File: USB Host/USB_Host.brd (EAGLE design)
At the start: 35 x 64 mm, 6 parts, among them J3 DIN5, X1 PG203J

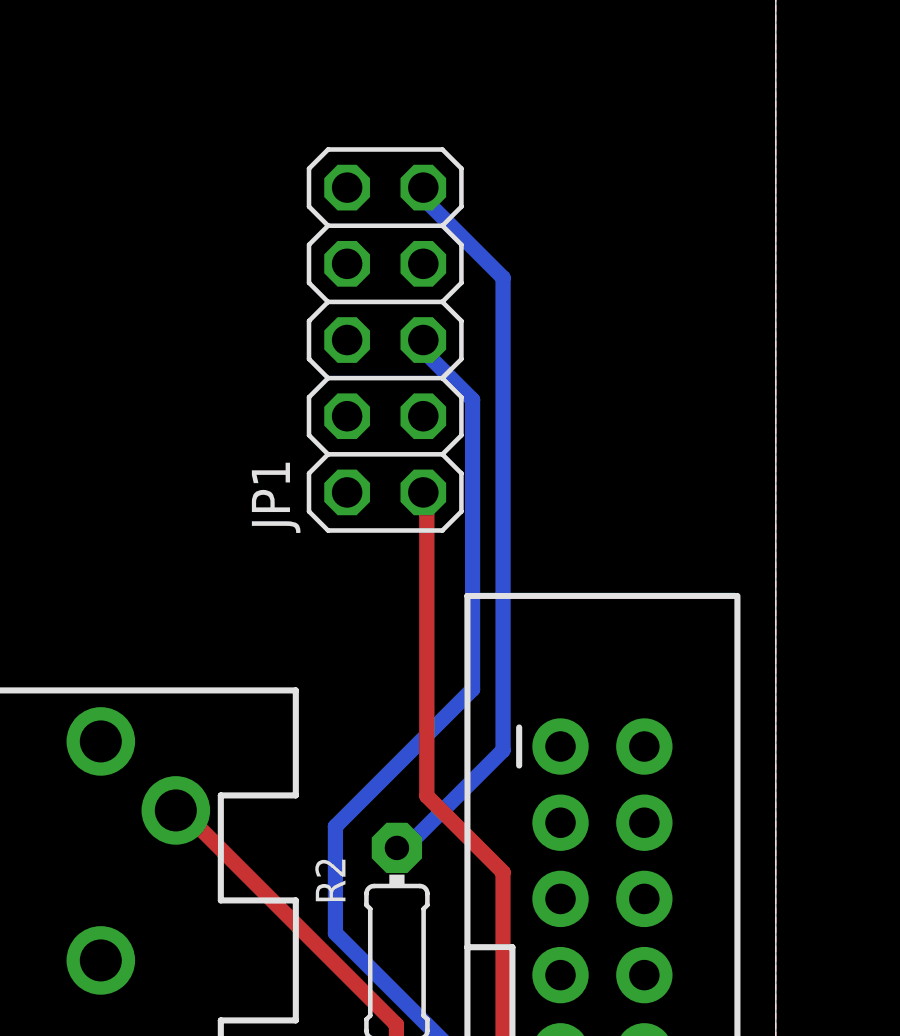
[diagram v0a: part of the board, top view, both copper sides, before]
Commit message: Adjustments to PCB Signed-off-by: goslo <digit99@mailinator.com>
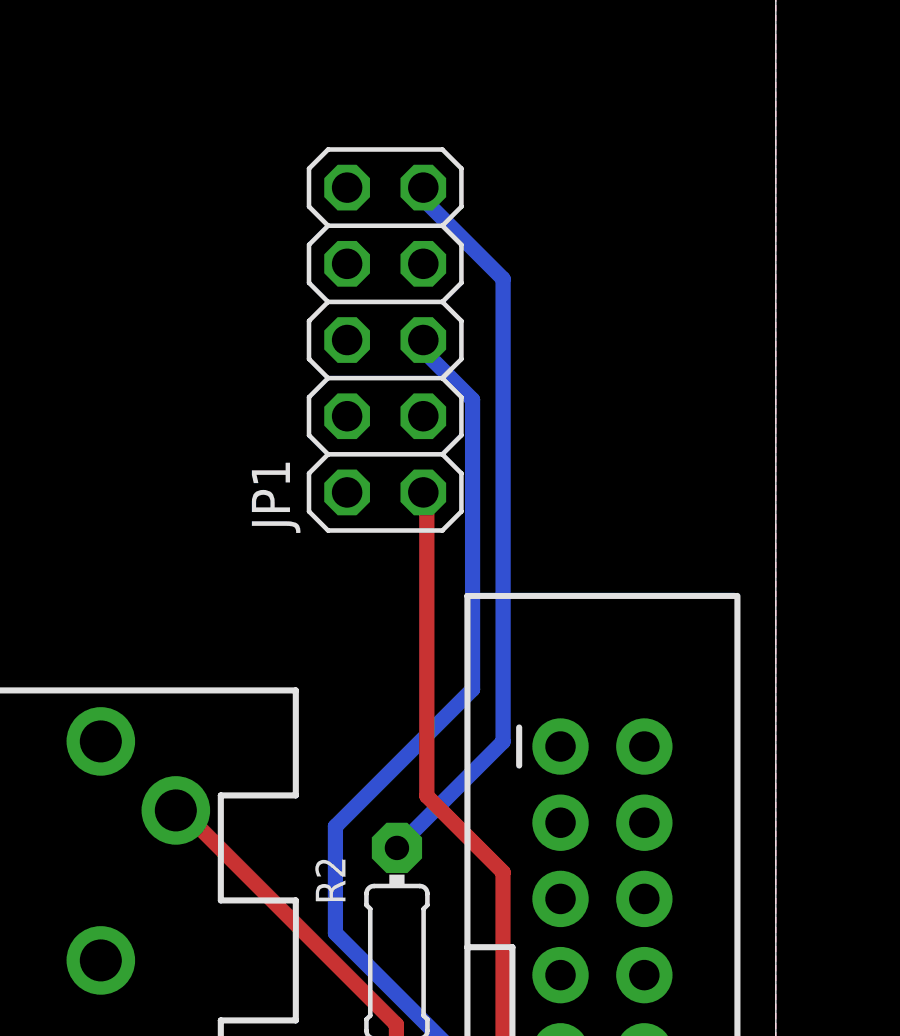
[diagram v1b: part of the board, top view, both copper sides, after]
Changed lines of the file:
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@@
 <signal name="GND">
 <contactref element="J3" pad="2"/>
-<polygon width="0" layer="16">
+<polygon width="0.5" layer="16">
 <vertex x="0" y="64"/>
 <vertex x="0" y="0"/>
@@
 <vertex x="35" y="64"/>
 </polygon>
-<polygon width="0" layer="1">
+<polygon width="0.5" layer="1">
 <vertex x="0" y="64"/>
 <vertex x="0" y="0"/>
@@
 <wire x1="27.94" y1="19.304" x2="27.823" y2="19.43" width="0.508" layer="1"/>
 </signal>
-<signal name="N$2">
+<signal name="N$1">
+<contactref element="JP1" pad="9"/>
 <contactref element="R2" pad="1"/>
-<contactref element="JP1" pad="9"/>
-<wire x1="25.908" y1="47.752" x2="23.368" y2="50.292" width="0.508" layer="16"/>
-<wire x1="25.908" y1="32.004" x2="25.908" y2="47.752" width="0.508" layer="16"/>
-<wire x1="22.86" y1="28.956" x2="25.908" y2="32.004" width="0.508" layer="16"/>
-<wire x1="23.368" y1="50.292" x2="23.25" y2="50.76" width="0.508" layer="16"/>
-<wire x1="22.86" y1="28.956" x2="22.37" y2="28.75" width="0.508" layer="16"/>
+<wire x1="23.25" y1="50.3752625" x2="23.25" y2="50.76" width="0.508" layer="16"/>
+<wire x1="25.908" y1="32.288" x2="25.908" y2="47.7172625" width="0.508" layer="16"/>
+<wire x1="25.908" y1="47.7172625" x2="23.25" y2="50.3752625" width="0.508" layer="16"/>
+<wire x1="22.37" y1="28.75" x2="25.908" y2="32.288" width="0.508" layer="16"/>
 </signal>
 </signals>
